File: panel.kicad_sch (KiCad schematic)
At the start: 7 parts, among them J13 Conn_01x06_Pin

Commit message: MPN BOOT BUTTON MINOR CHANGES
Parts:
- D11, D12, D13: footprint (none) -> LED_THT:LED_D5.0mm; MPN (none) -> 333-2SURD/S530-A3
- R46, R47, R48: MPN (none) -> 0805W8F2700T5E
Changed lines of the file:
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@@
+			)
+		)
+		(property "MPN" "0805W8F2700T5E"
+			(at 43.18 26.67 0)
+			(hide yes)
+			(show_name no)
+			(do_not_autoplace no)
+			(effects
+				(font
+					(size 1.27 1.27)
+				)
 			)
 		)
@@
 			)
 		)
+		(property "MPN" "0805W8F2700T5E"
+			(at 19.05 26.67 0)
+			(hide yes)
+			(show_name no)
+			(do_not_autoplace no)
+			(effects
+				(font
+					(size 1.27 1.27)
+				)
+			)
+		)
 		(pin "2"
 		)
@@
 			)
 		)
-		(property "Footprint" ""
+		(property "Footprint" "LED_THT:LED_D5.0mm"
 			(at 43.18 34.29 0)
 			(hide yes)
@@
 		)
 		(property "Sim.Pins" "1=K 2=A"
+			(at 43.18 34.29 0)
+			(hide yes)
+			(show_name no)
+			(do_not_autoplace no)
+			(effects
+				(font
+					(size 1.27 1.27)
+				)
+			)
+		)
+		(property "MPN" "333-2SURD/S530-A3"
 			(at 43.18 34.29 0)
 			(hide yes)
@@
 			)
 		)
-		(property "Footprint" ""
+		(property "Footprint" "LED_THT:LED_D5.0mm"
 			(at 31.75 34.29 0)
 			(hide yes)
@@
 		)
 		(property "Sim.Pins" "1=K 2=A"
+			(at 31.75 34.29 0)
+			(hide yes)
+			(show_name no)
+			(do_not_autoplace no)
+			(effects
+				(font
+					(size 1.27 1.27)
+				)
+			)
+		)
+		(property "MPN" "333-2SURD/S530-A3"
 			(at 31.75 34.29 0)
 			(hide yes)
@@
 			)
 		)
+		(property "MPN" "0805W8F2700T5E"
+			(at 31.75 26.67 0)
+			(hide yes)
+			(show_name no)
+			(do_not_autoplace no)
+			(effects
+				(font
+					(size 1.27 1.27)
+				)
+			)
+		)
 		(pin "2"
 		)
@@
 			)
 		)
-		(property "Footprint" ""
+		(property "Footprint" "LED_THT:LED_D5.0mm"
 			(at 19.05 34.29 0)
 			(hide yes)
@@
 			(at 19.05 34.29 0)
 			(hide yes)
+			(show_name no)
+			(do_not_autoplace no)
+			(effects
+				(font
+					(size 1.27 1.27)
+				)
+			)
+		)
+		(property "MPN" "333-2SURD/S530-A3"
+			(at 19.05 34.29 0)
+			(hide yes)

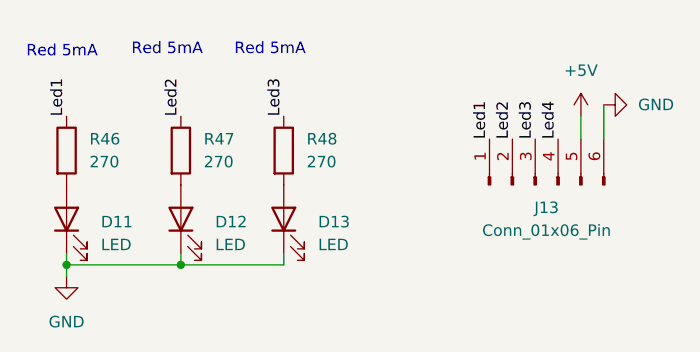
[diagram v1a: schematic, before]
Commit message: FINAL SCHEMATIC
Global nets, more ESD safety, complete bom, outlets, other fixes, ERC CLEAN
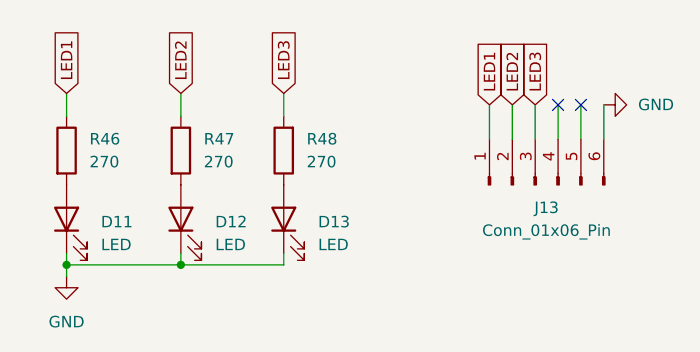
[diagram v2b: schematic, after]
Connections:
- net at D13.2 (A): now also R48.1; no longer R48.2
- net +5V: no longer names the net of J13.5 (Pin_5)
- net Led1 renamed LED1
- net Led2 renamed LED2
- net Led3 renamed LED3
- net LED3: now also R48.2; no longer R48.1
- net Led4: no longer names the net of J13.4 (Pin_4)
- no-connect marks 0 -> 2
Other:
- note removed: "Red 5mA"
- moved on the sheet: R48
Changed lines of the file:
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@@
 	(generator_version "10.0")
 	(paper "A4")
-	(text "Red 5mA\n"
-		(exclude_from_sim no)
-		(at 30.226 15.494 0)
-		(effects
-			(font
-				(size 1.27 1.27)
-			)
-		)
-	)
-	(text "Red 5mA\n"
-		(exclude_from_sim no)
-		(at 18.542 15.748 0)
-		(effects
-			(font
-				(size 1.27 1.27)
-			)
-		)
-	)
-	(text "Red 5mA\n"
-		(exclude_from_sim no)
-		(at 41.656 15.494 0)
-		(effects
-			(font
-				(size 1.27 1.27)
-			)
-		)
-	)
 	(junction
 		(at 31.75 39.37)
@@
 		(color 0 0 0 0)
 	)
+	(no_connect
+		(at 76.2 21.59)
+	)
+	(no_connect
+		(at 73.66 21.59)
+	)
 	(wire
 		(pts
@@
 	(wire
 		(pts
-			(xy 76.2 22.86) (xy 76.2 25.4)
+			(xy 43.18 20.32) (xy 43.18 22.86)
+		)
+		(stroke
+			(width 0)
+			(type default)
+		)
+	)
+	(wire
+		(pts
+			(xy 76.2 21.59) (xy 76.2 25.4)
+		)
+		(stroke
+			(width 0)
+			(type default)
+		)
+	)
+	(wire
+		(pts
+			(xy 19.05 20.32) (xy 19.05 22.86)
+		)
+		(stroke
+			(width 0)
+			(type default)
+		)
+	)
+	(wire
+		(pts
+			(xy 73.66 21.59) (xy 73.66 25.4)
+		)
+		(stroke
+			(width 0)
+			(type default)
+		)
+	)
+	(wire
+		(pts
+			(xy 71.12 21.59) (xy 71.12 25.4)
+		)
+		(stroke
+			(width 0)
+			(type default)
+		)
+	)
+	(wire
+		(pts
+			(xy 68.58 21.59) (xy 68.58 25.4)
 		)
 		(stroke
@@
 	(wire
 		(pts
+			(xy 66.04 21.59) (xy 66.04 25.4)
+		)
+		(stroke
+			(width 0)
+			(type default)
+		)
+	)
+	(wire
+		(pts
+			(xy 31.75 20.32) (xy 31.75 22.86)
+		)
+		(stroke
+			(width 0)
+			(type default)
+		)
+	)
+	(wire
+		(pts
 			(xy 31.75 39.37) (xy 43.18 39.37)
 		)
@@
 		)
 	)
-	(label "Led2"
-		(at 68.58 25.4 90)
+	(global_label "LED2"
+		(shape input)
+		(at 31.75 20.32 90)
+		(fields_autoplaced yes)
 		(effects
 			(font
 				(size 1.27 1.27)
 			)
-			(justify left bottom)
-		)
-	)
-	(label "Led3"
-		(at 43.18 22.86 90)
+			(justify left)
+		)
+		(property "Intersheetrefs" "${INTERSHEET_REFS}"
+			(at 31.75 13.3324 90)
+			(hide yes)
+			(show_name no)
+			(do_not_autoplace no)
+			(effects
+				(font
+					(size 1.27 1.27)
+				)
+				(justify left)
+			)
+		)
+	)
+	(global_label "LED1"
+		(shape input)
+		(at 19.05 20.32 90)
+		(fields_autoplaced yes)
 		(effects
 			(font
 				(size 1.27 1.27)
 			)
-			(justify left bottom)
-		)
-	)
-	(label "Led3"
-		(at 71.12 25.4 90)
+			(justify left)
+		)
+		(property "Intersheetrefs" "${INTERSHEET_REFS}"
+			(at 19.05 13.3324 90)
+			(hide yes)
+			(show_name no)
+			(do_not_autoplace no)
+			(effects
+				(font
+					(size 1.27 1.27)
+				)
+				(justify left)
+			)
+		)
+	)
+	(global_label "LED3"
+		(shape input)
+		(at 71.12 21.59 90)
+		(fields_autoplaced yes)
 		(effects
 			(font
 				(size 1.27 1.27)
 			)
-			(justify left bottom)
-		)
-	)
-	(label "Led2"
-		(at 31.75 22.86 90)
+			(justify left)
+		)
+		(property "Intersheetrefs" "${INTERSHEET_REFS}"
+			(at 71.12 14.6024 90)
+			(hide yes)
+			(show_name no)
+			(do_not_autoplace no)
+			(effects
+				(font
+					(size 1.27 1.27)
+				)
+				(justify left)
+			)
+		)
+	)
+	(global_label "LED3"
+		(shape input)
+		(at 43.18 20.32 90)
+		(fields_autoplaced yes)
 		(effects
 			(font
 				(size 1.27 1.27)
 			)
-			(justify left bottom)
-		)
-	)
-	(label "Led4"
-		(at 73.66 25.4 90)
+			(justify left)
+		)
+		(property "Intersheetrefs" "${INTERSHEET_REFS}"
+			(at 43.18 13.3324 90)
+			(hide yes)
+			(show_name no)
+			(do_not_autoplace no)
+			(effects
+				(font
+					(size 1.27 1.27)
+				)
+				(justify left)
+			)
+		)
+	)
+	(global_label "LED1"
+		(shape input)
+		(at 66.04 21.59 90)
+		(fields_autoplaced yes)
 		(effects
 			(font
 				(size 1.27 1.27)
 			)
-			(justify left bottom)
-		)
-	)
-	(label "Led1"
-		(at 19.05 22.86 90)
+			(justify left)
+		)
+		(property "Intersheetrefs" "${INTERSHEET_REFS}"
+			(at 66.04 14.6024 90)
+			(hide yes)
+			(show_name no)
+			(do_not_autoplace no)
+			(effects
+				(font
+					(size 1.27 1.27)
+				)
+				(justify left)
+			)
+		)
+	)
+	(global_label "LED2"
+		(shape input)
+		(at 68.58 21.59 90)
+		(fields_autoplaced yes)
 		(effects
 			(font
 				(size 1.27 1.27)
 			)
-			(justify left bottom)
-		)
-	)
-	(label "Led1"
-		(at 66.04 25.4 90)
-		(effects
-			(font
-				(size 1.27 1.27)
-			)
-			(justify left bottom)
+			(justify left)
+		)
+		(property "Intersheetrefs" "${INTERSHEET_REFS}"
+			(at 68.58 14.6024 90)
+			(hide yes)
+			(show_name no)
+			(do_not_autoplace no)
+			(effects
+				(font
+					(size 1.27 1.27)
+				)
+				(justify left)
+			)
 		)
 	)
 	(symbol
 		(lib_id "Device:R")
-		(at 43.18 26.67 0)
+		(at 43.18 26.67 180)
 		(unit 1)
 		(body_style 1)
@@
 					(size 1.27 1.27)
 				)
-				(justify left)
+				(justify right)
 			)
 		)
@@
 					(size 1.27 1.27)
 				)
-				(justify left)
+				(justify right)
 			)
 		)
 		(property "Footprint" "Resistor_SMD:R_0805_2012Metric"
-			(at 41.402 26.67 90)
+			(at 44.958 26.67 90)
 			(hide yes)
 			(show_name no)
@@
 					(unit 1)
 				)
-			)
-		)
-	)
-	(symbol
-		(lib_id "power:+3.3V")
-		(at 76.2 22.86 0)
-		(unit 1)
-		(body_style 1)
-		(exclude_from_sim no)
-		(in_bom yes)
-		(on_board yes)
-		(in_pos_files yes)
-		(dnp no)
-		(fields_autoplaced yes)
-		(property "Reference" "#PWR032"
-			(at 76.2 26.67 0)
-			(hide yes)
-			(show_name no)
-			(do_not_autoplace no)
-			(effects
-				(font
-					(size 1.27 1.27)
-				)
-			)
-		)
-		(property "Value" "+5V"
-			(at 76.2 17.78 0)
-			(show_name no)
-			(do_not_autoplace no)
-			(effects
-				(font
-					(size 1.27 1.27)
-				)
-			)
-		)
-		(property "Footprint" "Package_DFN_QFN:Diodes_UDFN3810-9_TYPE_B"
-			(at 76.2 22.86 0)
-			(hide yes)
-			(show_name no)
-			(do_not_autoplace no)
-			(effects
-				(font
-					(size 1.27 1.27)
-				)
-			)
-		)
-		(property "Datasheet" ""
-			(at 76.2 22.86 0)
-			(hide yes)
-			(show_name no)
-			(do_not_autoplace no)
-			(effects
-				(font
-					(size 1.27 1.27)
-				)
-			)
-		)
-		(property "Description" "Power symbol creates a global label with name \"+3.3V\""
-			(at 76.2 22.86 0)
-			(hide yes)
-			(show_name no)
-			(do_not_autoplace no)
-			(effects
-				(font
-					(size 1.27 1.27)
-				)
-			)
-		)
-		(pin "1"
-		)
-		(instances
-			(project "smart_supply"
-				(path "/487ef637-7a03-4925-80c1-798e0c6f0bbd/2c9929a5-2c00-45f1-baca-5f3ca7d07447"
-					(reference "#PWR032")
-					(unit 1)
-				)
